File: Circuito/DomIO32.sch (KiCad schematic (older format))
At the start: 51 parts, among them J2 Conector 1x5, J3 OSTTC032162, J4 OSTTC032162, J5 Conector 2x5, SW1 TactSwitch, U1 LM1117-3.3, U2 PIC32MM0064GPL028-I-SS, U3 ESP-02, X1 X, X2 X, X3 X

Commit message: Se corrige capacitor electrolitico para nuevas librerias
Se corrige capacitor electrolitico para nuevas librerias
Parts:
- C10, C14, C3: symbol Device:CP -> Device:C_Polarized
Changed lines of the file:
@@
 $EndComp
 $Comp
-L Device:CP C10
+L Device:C_Polarized C10
 U 1 1 5DCB76F2
 P 5600 4550
@@
 	5150 7250 5150 7100
 $Comp
-L Device:CP C3
+L Device:C_Polarized C3
 U 1 1 5DD06DD2
 P 3600 1700
@@
 $EndComp
 $Comp
-L Device:CP C14
+L Device:C_Polarized C14
 U 1 1 5ED72089
 P 2500 1700

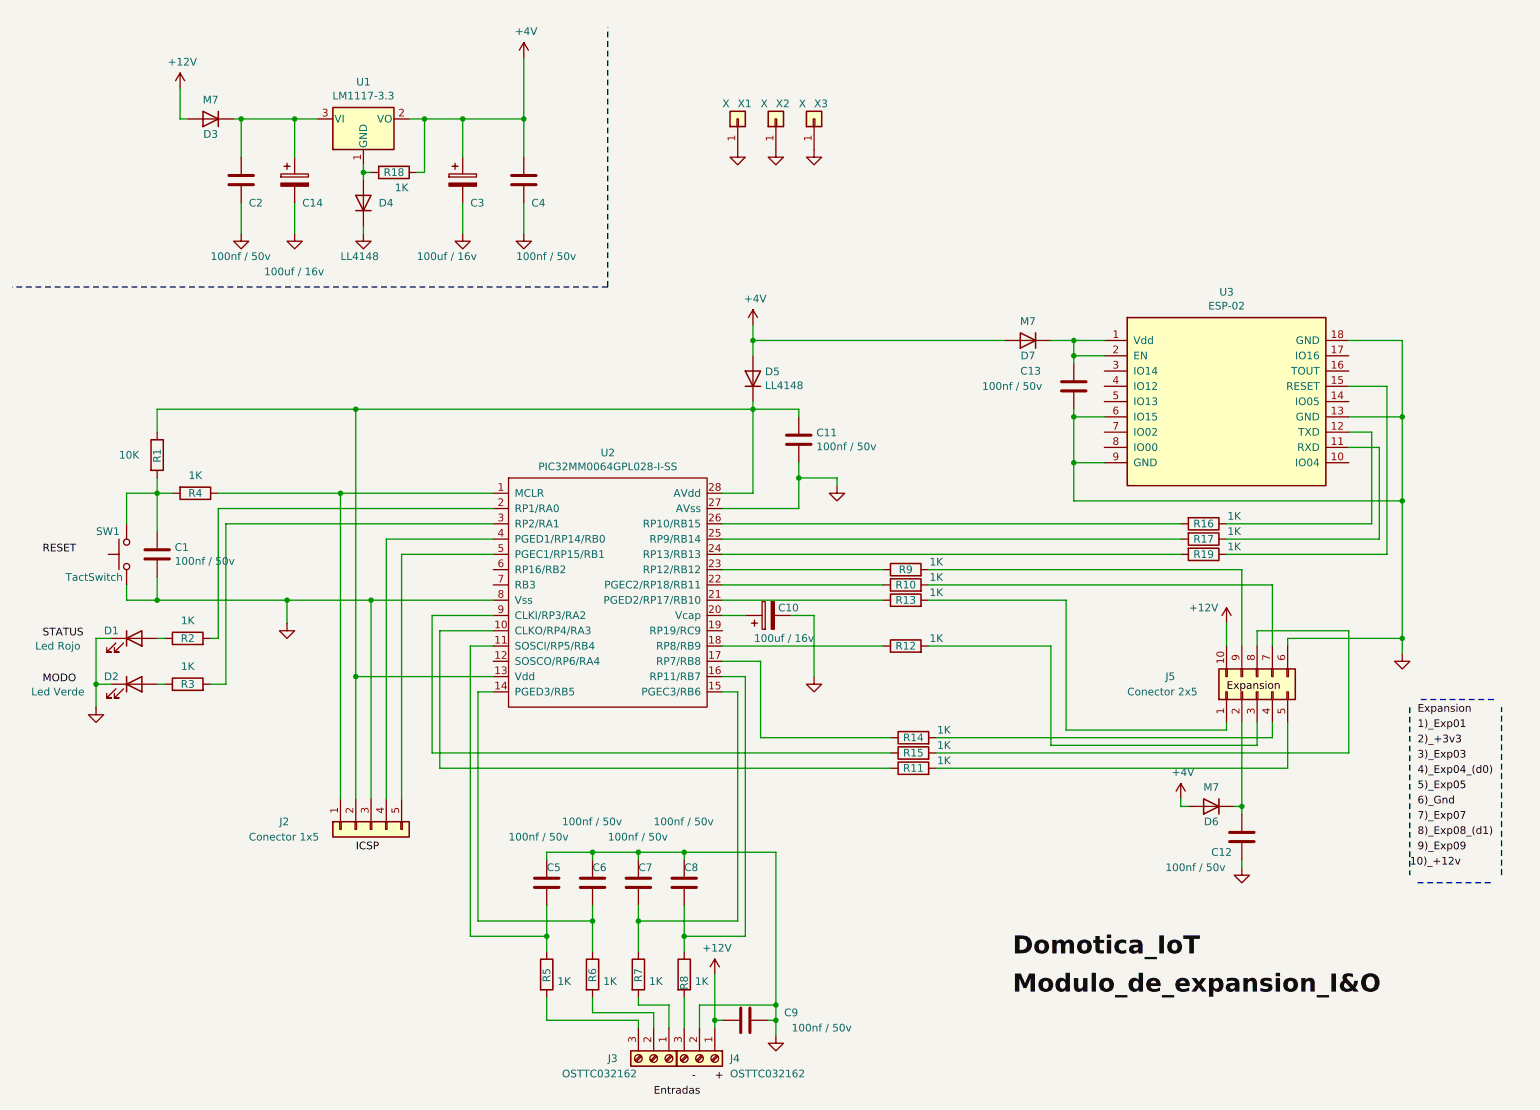
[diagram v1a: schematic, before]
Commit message: Cambio de planes
Cambio de planes
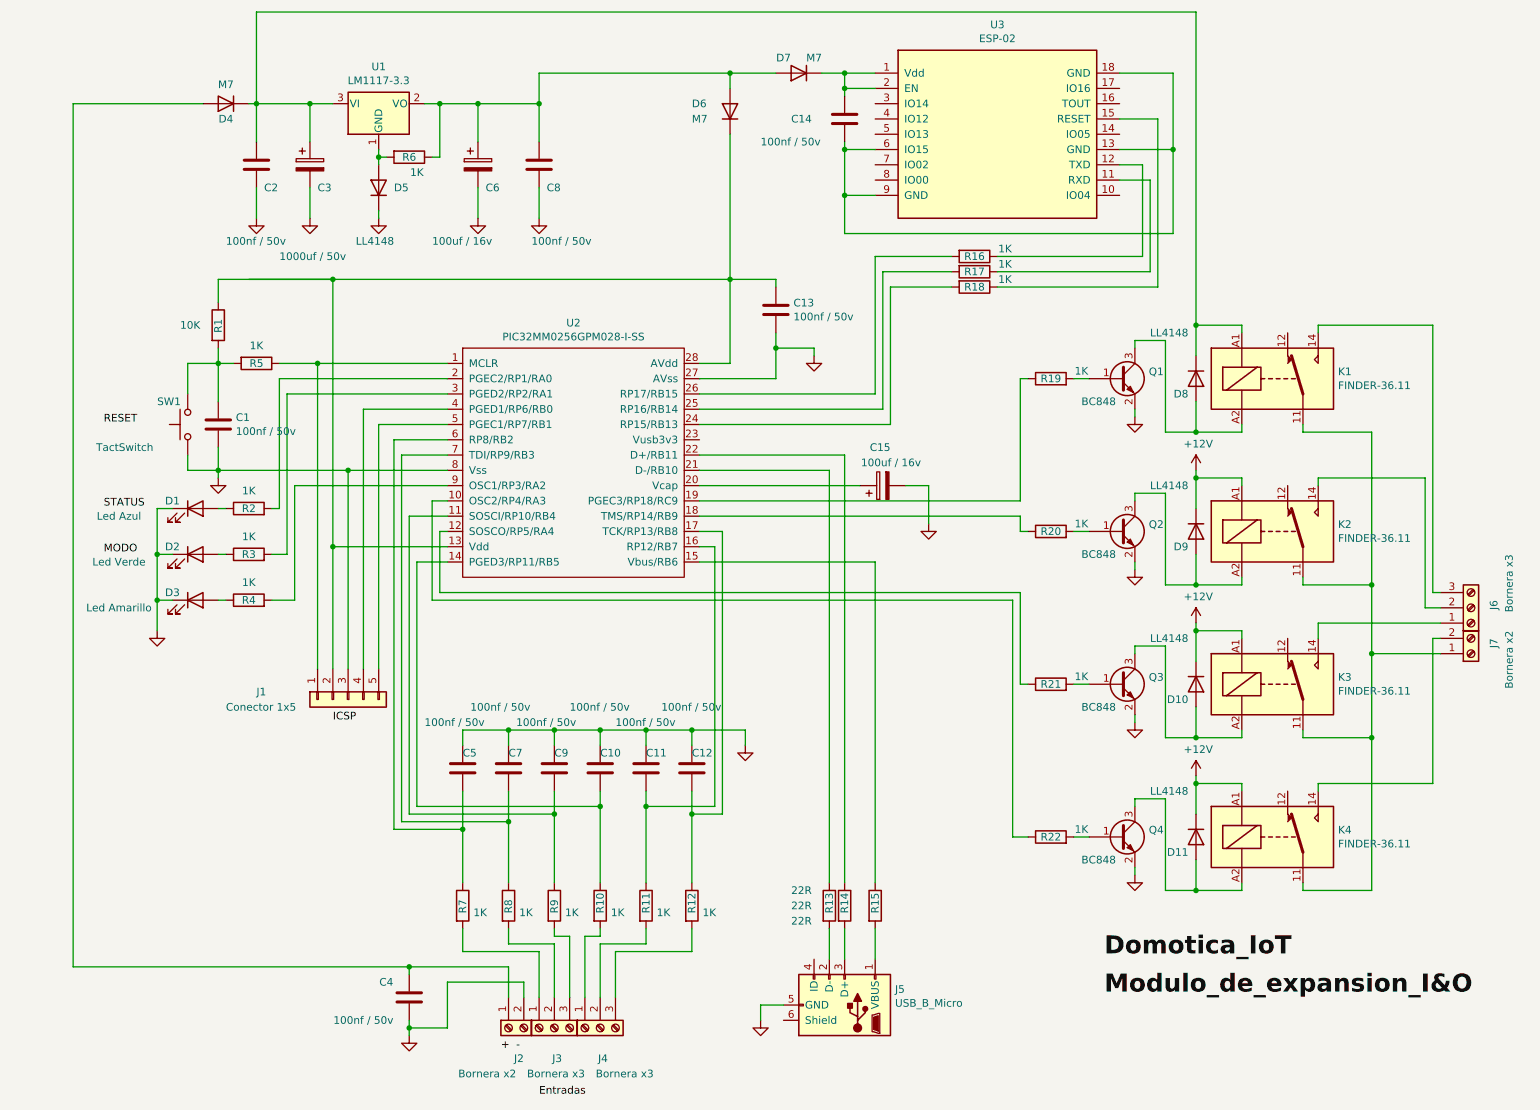
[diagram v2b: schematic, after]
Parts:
- removed C12: 100nf / 50v, Capacitor_SMD:C_0805_2012Metric_Pad1.15x1.40mm_HandSolder, symbol Device:C
- removed D6: M7, Diode_SMD:D_SMA, symbol Device:D
- removed J5: Conector 2x5, symbol Connector_Generic:Conn_02x05_Counter_Clockwise
- removed R10, R11, R12, R9: 1K, Resistor_SMD:R_0805_2012Metric_Pad1.15x1.40mm_HandSolder, symbol Device:R
- removed U2: PIC32MM0064GPL028-I-SS, Package_SO:SSOP-28_5.3x10.2mm_P0.65mm, symbol DomIO32-rescue:PIC32MM0064GPL028-I-SO-DomIO32
- removed X1, X2, X3: X, MountingHole:MountingHole_3.5mm_Pad, symbol Connector_Generic:Conn_01x01
- added C5, C7: 100nf / 50v, Capacitor_SMD:C_0805_2012Metric_Pad1.18x1.45mm_HandSolder, symbol Device:C
- added D10, D11, D8, D9: LL4148, Diode_SMD:D_SOD-128, symbol Device:D
- added D3: Led Amarillo, Diode_SMD:D_0805_2012Metric_Pad1.15x1.40mm_HandSolder, symbol Device:LED
- added J2, J7: Bornera x2, TerminalBlock_Phoenix:TerminalBlock_Phoenix_PT-1,5-2-5.0-H_1x02_P5.00mm_Horizontal, symbol Connector:Screw_Terminal_01x02
- added J5: USB_B_Micro, Connector_USB:USB_Micro-B_GCT_USB3076-30-A, symbol Connector:USB_B_Micro
- added J6: Bornera x3, TerminalBlock_Phoenix:TerminalBlock_Phoenix_PT-1,5-3-5.0-H_1x03_P5.00mm_Horizontal, symbol Connector:Screw_Terminal_01x03
- added K1, K2, K3, K4: FINDER-36.11, Relay_THT:Relay_SPDT_Finder_36.11, symbol Relay:FINDER-36.11
- added Q1, Q2, Q3, Q4: BC848, Package_TO_SOT_SMD:SOT-23, symbol Device:Q_NPN_BEC
- added R19, R20, R21, R22, R4, R7, R8: 1K, Resistor_SMD:R_0805_2012Metric_Pad1.20x1.40mm_HandSolder, symbol Device:R
- added U2: PIC32MM0256GPM028-I-SS, Package_SO:SSOP-28_5.3x10.2mm_P0.65mm, symbol DomIO32:PIC32MM0256GPM028-I-SS
- C1, C2: footprint Capacitor_SMD:C_0805_2012Metric_Pad1.15x1.40mm_HandSolder -> Capacitor_SMD:C_0805_2012Metric_Pad1.18x1.45mm_HandSolder
- C10: renamed from C6; footprint Capacitor_SMD:C_0805_2012Metric_Pad1.15x1.40mm_HandSolder -> Capacitor_SMD:C_0805_2012Metric_Pad1.18x1.45mm_HandSolder
- C11: renamed from C7; footprint Capacitor_SMD:C_0805_2012Metric_Pad1.15x1.40mm_HandSolder -> Capacitor_SMD:C_0805_2012Metric_Pad1.18x1.45mm_HandSolder
- C12: renamed from C8; footprint Capacitor_SMD:C_0805_2012Metric_Pad1.15x1.40mm_HandSolder -> Capacitor_SMD:C_0805_2012Metric_Pad1.18x1.45mm_HandSolder
- C13: renamed from C11; footprint Capacitor_SMD:C_0805_2012Metric_Pad1.15x1.40mm_HandSolder -> Capacitor_SMD:C_0805_2012Metric_Pad1.18x1.45mm_HandSolder
- C14: renamed from C13; footprint Capacitor_SMD:C_0805_2012Metric_Pad1.15x1.40mm_HandSolder -> Capacitor_SMD:C_0805_2012Metric_Pad1.18x1.45mm_HandSolder
- C3: renamed from C14; value 100uf / 16v -> 1000uf / 50v; footprint Capacitor_THT:CP_Radial_D6.3mm_P2.50mm -> Capacitor_THT:CP_Radial_D8.0mm_P5.00mm
- C4: renamed from C9; footprint Capacitor_SMD:C_0805_2012Metric_Pad1.15x1.40mm_HandSolder -> Capacitor_SMD:C_0805_2012Metric_Pad1.18x1.45mm_HandSolder
- C8: renamed from C4; footprint Capacitor_SMD:C_0805_2012Metric_Pad1.15x1.40mm_HandSolder -> Capacitor_SMD:C_0805_2012Metric_Pad1.18x1.45mm_HandSolder
- C9: renamed from C5; footprint Capacitor_SMD:C_0805_2012Metric_Pad1.15x1.40mm_HandSolder -> Capacitor_SMD:C_0805_2012Metric_Pad1.18x1.45mm_HandSolder
- D1: value Led Rojo -> Led Azul
- D5: renamed from D4; footprint Diode_SMD:D_0805_2012Metric_Pad1.15x1.40mm_HandSolder -> Diode_SMD:D_SOD-128
- D6: renamed from D5; value LL4148 -> M7; footprint Diode_SMD:D_0805_2012Metric_Pad1.15x1.40mm_HandSolder -> Diode_SMD:D_SMA
- J3, J4: value OSTTC032162 -> Bornera x3
- R1, R16, R17, R2, R3: footprint Resistor_SMD:R_0805_2012Metric_Pad1.15x1.40mm_HandSolder -> Resistor_SMD:R_0805_2012Metric_Pad1.20x1.40mm_HandSolder
- R10: renamed from R6; footprint Resistor_SMD:R_0805_2012Metric_Pad1.15x1.40mm_HandSolder -> Resistor_SMD:R_0805_2012Metric_Pad1.20x1.40mm_HandSolder
- R11: renamed from R7; footprint Resistor_SMD:R_0805_2012Metric_Pad1.15x1.40mm_HandSolder -> Resistor_SMD:R_0805_2012Metric_Pad1.20x1.40mm_HandSolder
- R12: renamed from R8; footprint Resistor_SMD:R_0805_2012Metric_Pad1.15x1.40mm_HandSolder -> Resistor_SMD:R_0805_2012Metric_Pad1.20x1.40mm_HandSolder
- R13, R14, R15: value 1K -> 22R; footprint Resistor_SMD:R_0805_2012Metric_Pad1.15x1.40mm_HandSolder -> Resistor_SMD:R_0805_2012Metric_Pad1.20x1.40mm_HandSolder
- R18: renamed from R19; footprint Resistor_SMD:R_0805_2012Metric_Pad1.15x1.40mm_HandSolder -> Resistor_SMD:R_0805_2012Metric_Pad1.20x1.40mm_HandSolder
- R5: renamed from R4; footprint Resistor_SMD:R_0805_2012Metric_Pad1.15x1.40mm_HandSolder -> Resistor_SMD:R_0805_2012Metric_Pad1.20x1.40mm_HandSolder
- R6: renamed from R18; footprint Resistor_SMD:R_0805_2012Metric_Pad1.15x1.40mm_HandSolder -> Resistor_SMD:R_0805_2012Metric_Pad1.20x1.40mm_HandSolder
- R9: renamed from R5; footprint Resistor_SMD:R_0805_2012Metric_Pad1.15x1.40mm_HandSolder -> Resistor_SMD:R_0805_2012Metric_Pad1.20x1.40mm_HandSolder
- renumbered C10 to C15, C3 to C6, D3 to D4, J2 to J1
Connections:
- net +12V: now also D10.1 (K), D11.1 (K), D9.1 (K), K2.A1, K3.A1, K4.A1; no longer C4.2, D4.2 (A), J4.1 (Pin_1)
- net GND: now also C5.1, C7.1, D3.1 (K), J2.2 (Pin_2), J5.5 (GND), Q1.2 (E), Q2.2 (E), Q3.2 (E), Q4.2 (E), U2.27 (AVss), U2.8 (Vss); no longer C14.2, J4.2 (Pin_2), U3.13 (GND), U3.18 (GND), U3.6 (IO15), U3.9 (GND)
- net at C15.1: now also U2.20 (Vcap)
- net at J1.1 (Pin_1), R5.1: now also U2.1 (MCLR)
- net at C13.1, D6.1 (K), J1.2 (Pin_2)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: now also U2.13 (Vdd), U2.28 (AVdd)
- net at R16.2: now also U2.26 (RP17/RB15)
- net at R17.2: now also U2.25 (RP16/RB14)
- net at C9.2, R9.1: now also U2.11 (SOSCI/RP10/RB4)
- net at C10.2, R10.1: now also U2.14 (PGED3/RP11/RB5)
- net at C11.2, R11.1: now also U2.16 (RP12/RB7)
- net at C12.2, R12.1: now also U2.17 (TCK/RP13/RB8)
- net at R14.1: now also U2.22 (D+/RB11)
- net at R2.2: now also U2.2 (PGEC2/RP1/RA0)
- net at R13.1: now also U2.21 (D-/RB10)
- net at R18.2: now also U2.24 (RP15/RB13)
- net at R3.2: now also U2.3 (PGED2/RP2/RA1)
- net at J1.4 (Pin_4): now also U2.4 (PGED1/RP6/RB0)
- net at J1.5 (Pin_5): now also U2.5 (PGEC1/RP7/RB1)
- net at R15.1: now also U2.15 (Vbus/RB6)
- net at R10.2: now also J4.1 (Pin_1); no longer J3.2 (Pin_2)
- net at R11.2: now also J4.2 (Pin_2); no longer J3.1 (Pin_1)
- net at C2.1, C3.1, D4.1 (K)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: now also D8.1 (K), K1.A1
- net at R14.2: now also J5.3 (D+)
- net at R15.2: now also J5.1 (VBUS)
- net at R13.2: now also J5.2 (D-)
- net +4V: no longer names the net of C6.1, C8.1, D6.2 (A), D7.2 (A), R6.1, U1.2 (VO)
- new net: C14.2, U3.13 (GND), U3.18 (GND), U3.6 (IO15), U3.9 (GND)
- new net: C4.2, D4.2 (A), J2.1 (Pin_1)
- new net: J3.1 (Pin_1), R7.2
- new net: J3.2 (Pin_2), R8.2
- new net: J7.1 (Pin_1), K1.11, K2.11, K3.11, K4.11
- new net: J6.3 (Pin_3), K1.14
- new net: D8.2 (A), K1.A2, Q1.3 (C)
- new net: D3.2 (A), R4.1
- new net: R4.2, U2.9 (OSC1/RP3/RA2)
- new net: J6.2 (Pin_2), K2.14
- new net: D9.2 (A), K2.A2, Q2.3 (C)
- new net: J6.1 (Pin_1), K3.14
- new net: D10.2 (A), K3.A2, Q3.3 (C)
- new net: J7.2 (Pin_2), K4.14
- new net: D11.2 (A), K4.A2, Q4.3 (C)
- new net: R22.1, U2.10 (OSC2/RP4/RA3)
- new net: Q4.1 (B), R22.2
- new net: R21.1, U2.12 (SOSCO/RP5/RA4)
- new net: Q3.1 (B), R21.2
- new net: R20.1, U2.18 (TMS/RP14/RB9)
- new net: Q2.1 (B), R20.2
- new net: R19.1, U2.19 (PGEC3/RP18/RC9)
- new net: Q1.1 (B), R19.2
- new net: C5.2, R7.1, U2.6 (RP8/RB2)
- new net: C7.2, R8.1, U2.7 (TDI/RP9/RB3)
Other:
- moved on the sheet: C1, C10, C11, C12, C13, C14, C15, C2, C3, C4, C6, C8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

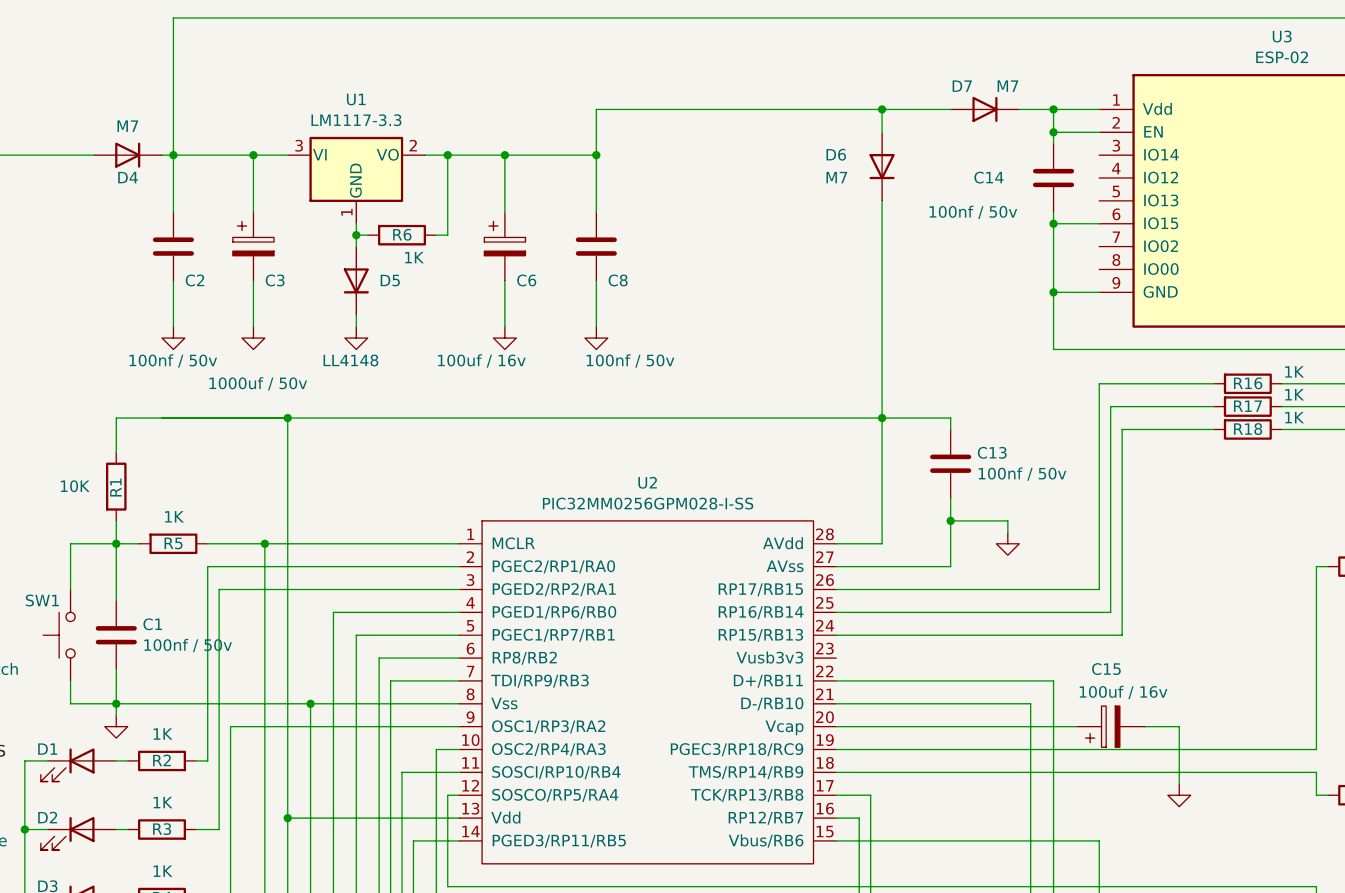
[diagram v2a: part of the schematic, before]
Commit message: Nuevo circuito co relees
Nuevo circuito co relees
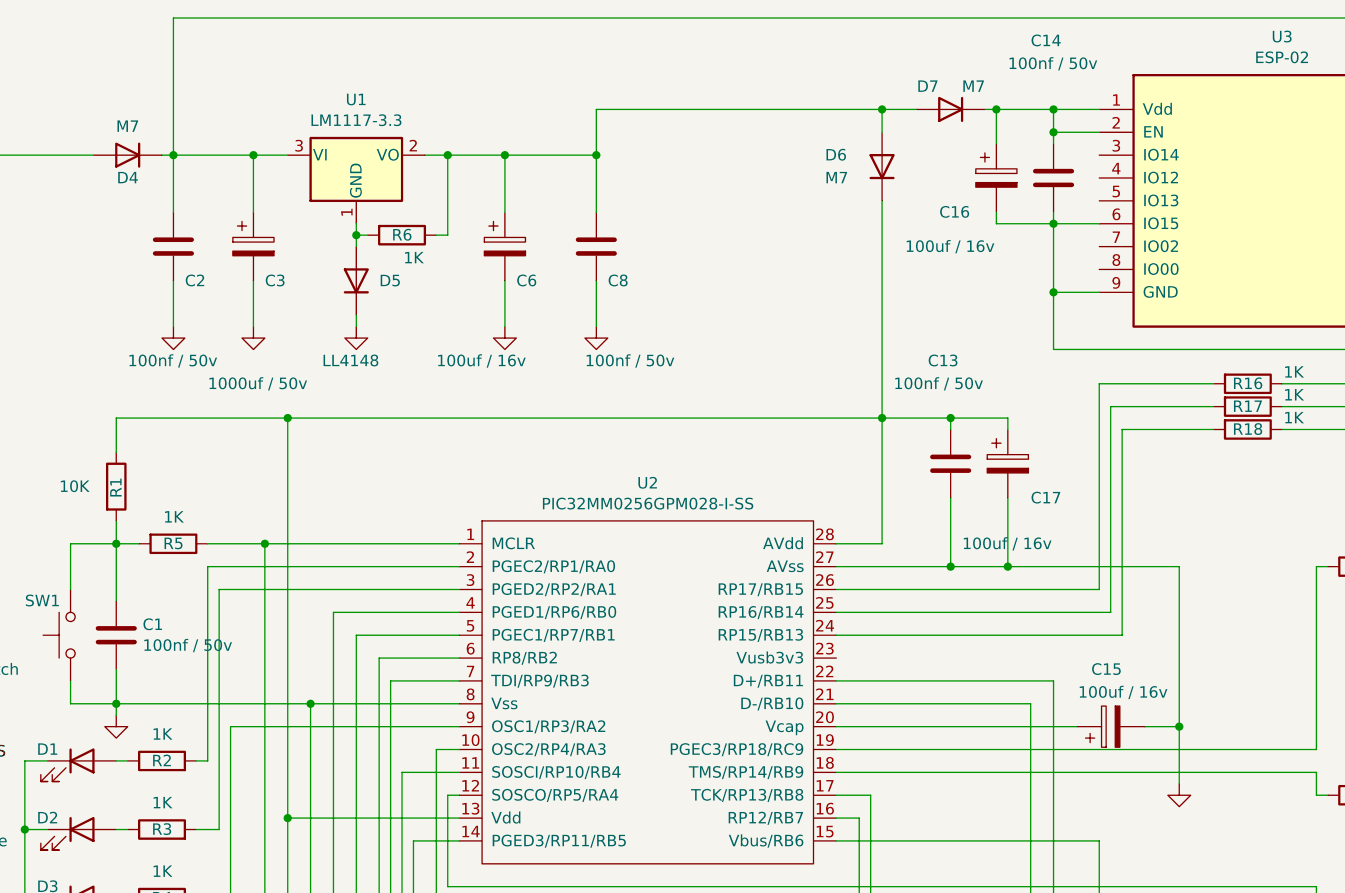
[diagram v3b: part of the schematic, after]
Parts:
- added C16, C17: 100uf / 16v, Capacitor_THT:CP_Radial_D6.3mm_P2.50mm, symbol Device:C_Polarized
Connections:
- net GND: now also C17.2
- net at C14.1, D7.1 (K), U3.1 (Vdd)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: now also C16.1
- net at C14.2, U3.13 (GND), U3.18 (GND)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: now also C16.2
- net at C13.1, D6.1 (K), J1.2 (Pin_2)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: now also C17.1
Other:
- moved on the sheet: D7
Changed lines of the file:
@@
 U 1 1 5DCDBCE7
 P 5650 2550
-F 0 "C13" H 5765 2596 50  0000 L CNN
-F 1 "100nf / 50v" H 5765 2505 50  0000 L CNN
+F 0 "C13" H 5550 3000 50  0000 L CNN
+F 1 "100nf / 50v" H 5400 2900 50  0000 L CNN
 F 2 "Capacitor_SMD:C_0805_2012Metric_Pad1.18x1.45mm_HandSolder" H 5688 2400 50  0001 C CNN
 F 3 "~" H 5650 2550 50  0001 C CNN
@@
 U 1 1 5DCDBD3D
 P 6100 1300
-F 0 "C14" H 5750 1300 50  0000 L CNN
-F 1 "100nf / 50v" H 5550 1150 50  0000 L CNN
+F 0 "C14" H 6000 1900 50  0000 L CNN
+F 1 "100nf / 50v" H 5900 1800 50  0000 L CNN
 F 2 "Capacitor_SMD:C_0805_2012Metric_Pad1.18x1.45mm_HandSolder" H 6138 1150 50  0001 C CNN
 F 3 "~" H 6100 1300 50  0001 C CNN
@@
 Wire Wire Line
 	3700 1200 4100 1200
-Wire Wire Line
-	5950 1000 6100 1000
 $Comp
 L Connector_Generic:Conn_01x05 J1
@@
 Wire Wire Line
 	5150 3000 5650 3000
-$Comp
-L power:GND #PWR011
-U 1 1 5DDE0DA2
-P 5900 2850
-F 0 "#PWR011" H 5900 2600 50  0001 C CNN
-F 1 "GND" H 5905 2677 50  0001 C CNN
-F 2 "" H 5900 2850 50  0001 C CNN
-F 3 "" H 5900 2850 50  0001 C CNN
-	1    5900 2850
-	1    0    0    -1
-$EndComp
 Wire Wire Line
 	5350 2350 5650 2350
 Wire Wire Line
 	5650 2350 5650 2400
-Wire Wire Line
-	5650 2700 5650 2800
-Wire Wire Line
-	5900 2850 5900 2800
-Wire Wire Line
-	5900 2800 5650 2800
-Connection ~ 5650 2800
-Wire Wire Line
-	5650 2800 5650 3000
 $Comp
 L Device:C C4
@@
 L Device:D D7
 U 1 1 5EE1D488
-P 5800 1000
-F 0 "D7" H 5900 900 50  0000 C CNN
-F 1 "M7" H 5700 900 50  0000 C CNN
-F 2 "Diode_SMD:D_SMA" H 5800 1000 50  0001 C CNN
-F 3 "~" H 5800 1000 50  0001 C CNN
-	1    5800 1000
+P 5650 1000
+F 0 "D7" H 5750 900 50  0000 C CNN
+F 1 "M7" H 5550 900 50  0000 C CNN
+F 2 "Diode_SMD:D_SMA" H 5650 1000 50  0001 C CNN
+F 3 "~" H 5650 1000 50  0001 C CNN
+	1    5650 1000
 	-1   0    0    1
 $EndComp
@@
 	2000 3650 2000 3600
 Wire Wire Line
-	5650 1000 5350 1000
-Wire Wire Line
 	5150 3100 6300 3100
 Wire Wire Line
@@
 Wire Wire Line
 	4100 1000 4100 1200
-Connection ~ 5350 1000
 Connection ~ 4100 1200
 $Comp
@@
 	8400 600  2250 600
 Wire Wire Line
-	2200 2350 2750 2350
-Wire Wire Line
 	2250 600  2250 1200
 Wire Wire Line
@@
 Wire Wire Line
 	2000 2350 2750 2350
+$Comp
+L Device:C_Polarized C16
+U 1 1 62189655
+P 5850 1300
+F 0 "C16" H 5600 1150 50  0000 L CNN
+F 1 "100uf / 16v" H 5450 1000 50  0000 L CNN
+F 2 "Capacitor_THT:CP_Radial_D6.3mm_P2.50mm" H 5888 1150 50  0001 C CNN
+F 3 "~" H 5850 1300 50  0001 C CNN
+	1    5850 1300
+	1    0    0    -1
+$EndComp
+Wire Wire Line
+	5500 1000 5350 1000
+Connection ~ 5350 1000
+Wire Wire Line
+	5800 1000 5850 1000
+Wire Wire Line
+	5850 1150 5850 1000
+Connection ~ 5850 1000
+Wire Wire Line
+	5850 1000 6100 1000
+Wire Wire Line
+	5850 1450 5850 1500
+Wire Wire Line
+	5850 1500 6100 1500
+Wire Wire Line
+	5650 2700 5650 3000
+Wire Wire Line
+	5650 3000 5900 3000
+Wire Wire Line
+	6650 3000 6650 3700
+Connection ~ 5650 3000
+Connection ~ 6650 3700
+$Comp
+L Device:C_Polarized C17
+U 1 1 6221BD48
+P 5900 2550
+F 0 "C17" H 6000 2400 50  0000 L CNN
+F 1 "100uf / 16v" H 5700 2200 50  0000 L CNN
+F 2 "Capacitor_THT:CP_Radial_D6.3mm_P2.50mm" H 5938 2400 50  0001 C CNN
+F 3 "~" H 5900 2550 50  0001 C CNN
+	1    5900 2550
+	1    0    0    -1
+$EndComp
+Wire Wire Line
+	5650 2350 5900 2350
+Wire Wire Line
+	5900 2350 5900 2400
+Connection ~ 5650 2350
+Wire Wire Line
+	5900 2700 5900 3000
+Connection ~ 5900 3000
+Wire Wire Line
+	5900 3000 6650 3000
 $EndSCHEMATC
